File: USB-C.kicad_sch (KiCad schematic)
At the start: 38 parts, among them IC2 TPS2557QDRBTQ1, IC5 TPS2557QDRBTQ1, IC7 TPS2557QDRBTQ1, J10 USB_C_Receptacle, J5 USB_C_Receptacle_USB2.0_16P, J7 USB_C_Receptacle_USB2.0_16P, U2 TPD1E05U06DYA, U3 TPD1E05U06DYA, U4 TPD1E05U06DYA

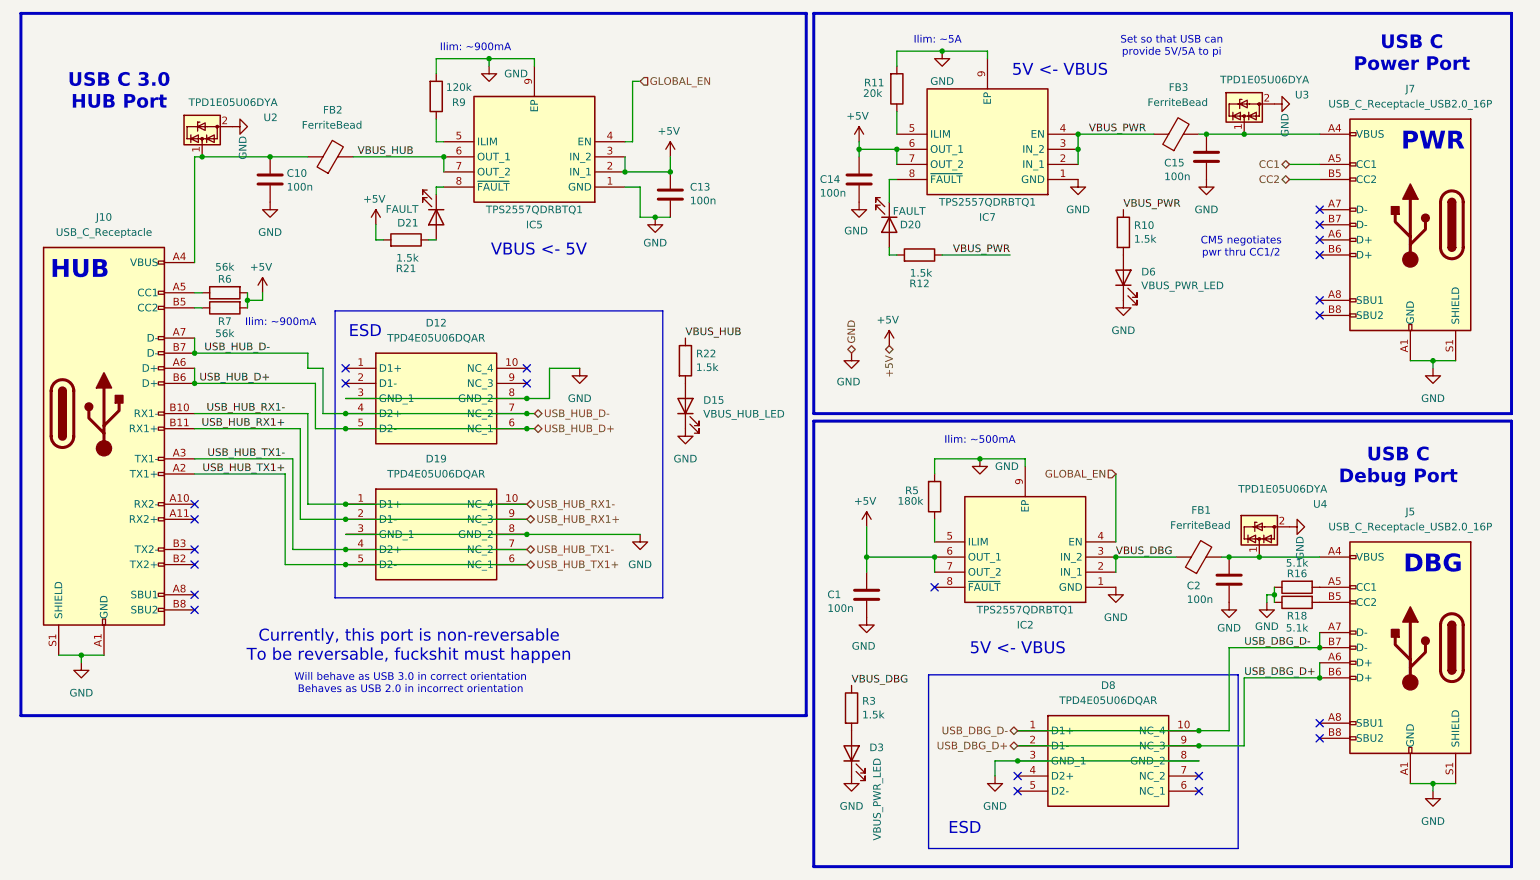
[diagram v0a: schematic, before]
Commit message: my life could not be worse right now
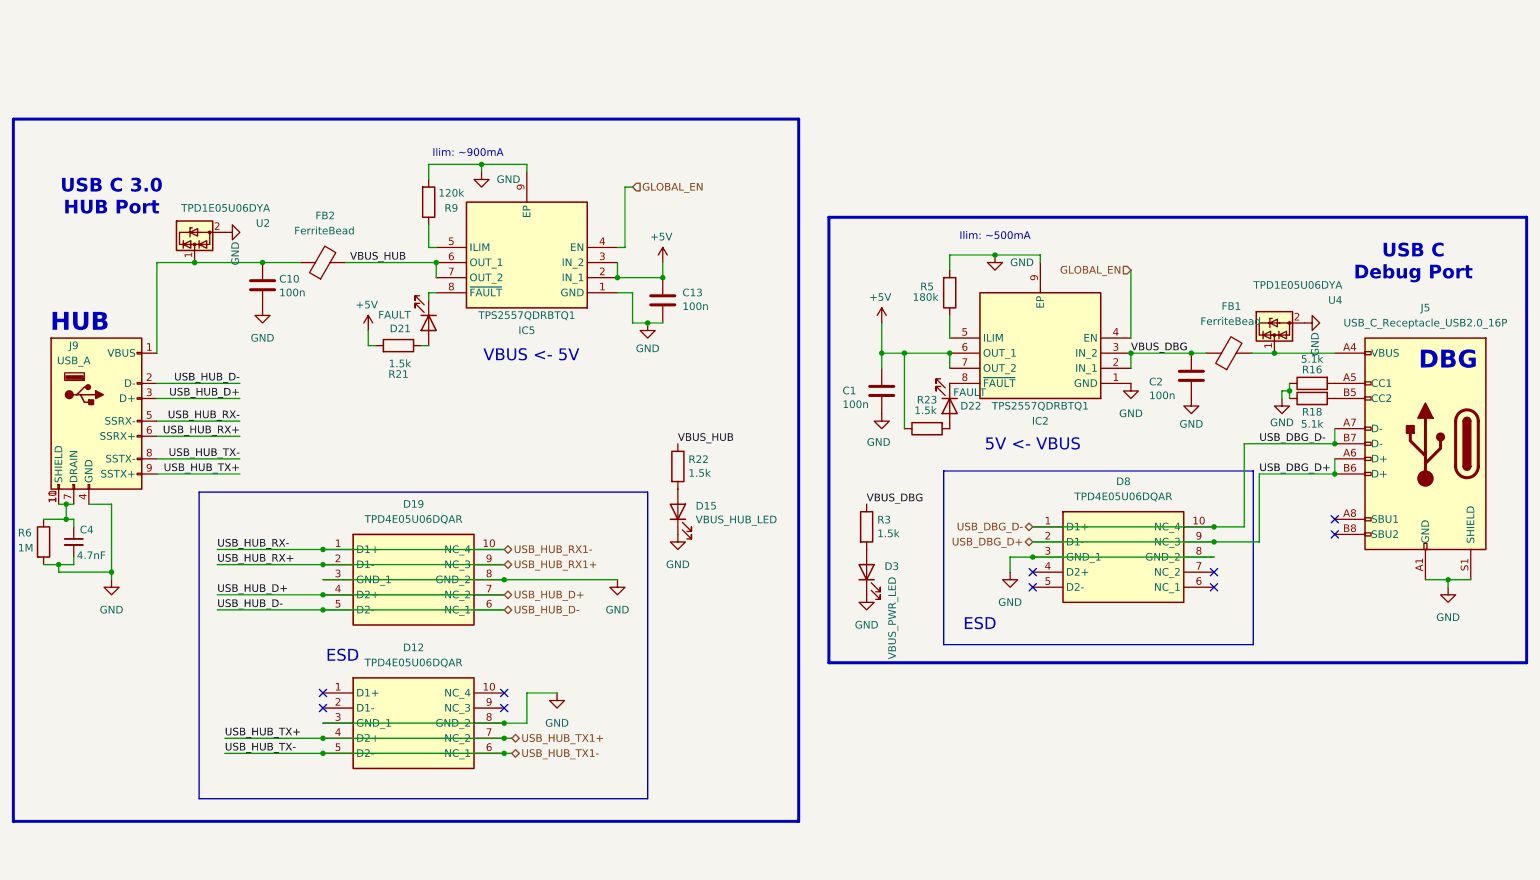
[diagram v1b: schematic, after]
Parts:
- removed C14, C15: 100n, Capacitor_SMD:C_0603_1608Metric_Pad1.08x0.95mm_HandSolder, symbol Device:C
- removed D20: FAULT, LED_SMD:LED_0603_1608Metric_Pad1.05x0.95mm_HandSolder, symbol Device:LED
- removed D6: VBUS_PWR_LED, LED_SMD:LED_0603_1608Metric_Pad1.05x0.95mm_HandSolder, symbol Device:LED
- removed FB3: FerriteBead, Inductor_SMD:L_1206_3216Metric, symbol Device:FerriteBead
- removed IC7: TPS2557QDRBTQ1, Controls_Pi:SON65P300X300X100-9N-D, symbol TPS2557QDRBTQ1:TPS2557QDRBTQ1
- removed J10: USB_C_Receptacle, Controls_Pi:CONN_221608-0001_MOL, symbol Connector:USB_C_Receptacle
- removed J7: USB_C_Receptacle_USB2.0_16P, Controls_Pi:2193200001, symbol Connector:USB_C_Receptacle_USB2.0_16P
- removed R10, R12: 1.5k, Resistor_SMD:R_0603_1608Metric_Pad0.98x0.95mm_HandSolder, symbol Device:R
- removed R11: 20k, Resistor_SMD:R_0603_1608Metric_Pad0.98x0.95mm_HandSolder, symbol Device:R
- removed R7: 56k, Resistor_SMD:R_0603_1608Metric_Pad0.98x0.95mm_HandSolder, symbol Device:R
- removed U3: TPD1E05U06DYA, Diode_SMD:D_SOD-523, symbol Power_Protection:TPD1E05U06DYA
- added C4: 4.7nF, Capacitor_SMD:C_0603_1608Metric_Pad1.08x0.95mm_HandSolder, symbol Device:C_Small
- added D22: FAULT, LED_SMD:LED_0603_1608Metric_Pad1.05x0.95mm_HandSolder, symbol Device:LED
- added J9: USB_A, Controls_Pi:CONN_484050003_MOL, symbol Connector:USB_A
- added R23: 1.5k, Resistor_SMD:R_0603_1608Metric_Pad0.98x0.95mm_HandSolder, symbol Device:R
- R6: value 56k -> 1M
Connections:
- net +5V: now also R23.1; no longer R6.2
- net GND: now also R6.2, C4.2, J9.4 (GND)
- net USB_HUB_D+: now also D19.4 (D2+), D19.7 (NC_2), J9.3 (D+); no longer D12.5 (D2-), D12.6 (NC_1)
- net USB_HUB_D-: now also D19.5 (D2-), D19.6 (NC_1), J9.2 (D-); no longer D12.4 (D2+), D12.7 (NC_2)
- net USB_HUB_RX1+: now also J9.6 (SSRX+)
- net USB_HUB_RX1-: now also J9.5 (SSRX-)
- net USB_HUB_TX1+: now also D12.4 (D2+), D12.7 (NC_2), J9.9 (SSTX+); no longer D19.5 (D2-), D19.6 (NC_1)
- net USB_HUB_TX1-: now also D12.5 (D2-), D12.6 (NC_1), J9.8 (SSTX-); no longer D19.4 (D2+), D19.7 (NC_2)
- net VBUS_DBG: now also C2.1
- net at C10.1, FB2.1, U2.1 (I/O): now also J9.1 (VBUS)
- net at FB1.2, J5.A4 (VBUS), J5.A9 (VBUS)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: no longer C2.1
- net at R6.1: now also C4.1, J9.10 (SHIELD), J9.11 (SHIELD), J9.7 (DRAIN)
- net at IC2.8 (~{FAULT}): now also D22.1 (K)
- new net: D22.2 (A), R23.2
- no-connect marks 23 -> 10
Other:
- note removed: "CM5 negotiates pwr thru CC1/2"
- note removed: "Currently, this port is non-reversable To be reversable, fuckshit must happen"
- note removed: "Ilim: ~5A"
- note removed: "PWR"
- note removed: "Set so that USB can provide 5V/5A to pi"
- note removed: "USB C Power Port"
- note removed: "Will behave as USB 3.0 in correct orientation Behaves as USB 2.0 in incorrect orientation"
- moved on the sheet: C1, C10, C13, C2, D12, D15, D19, D21, D3, D8, FB1, FB2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

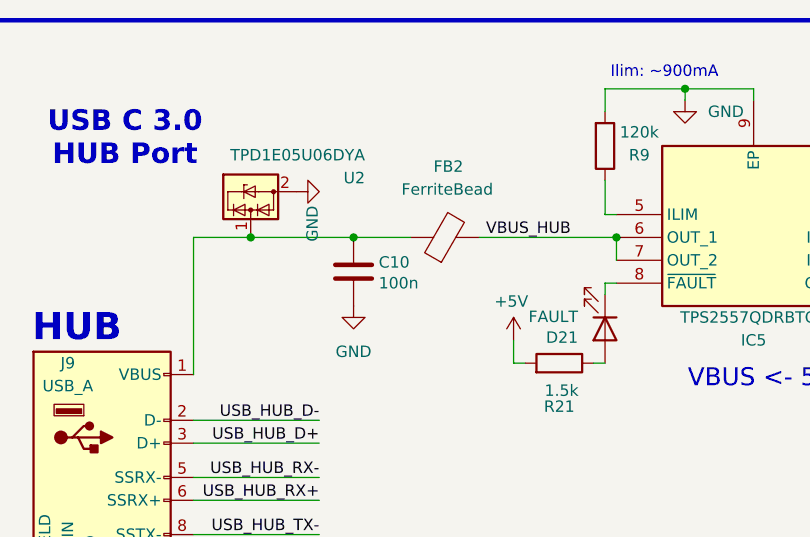
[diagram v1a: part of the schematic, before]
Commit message: frink2
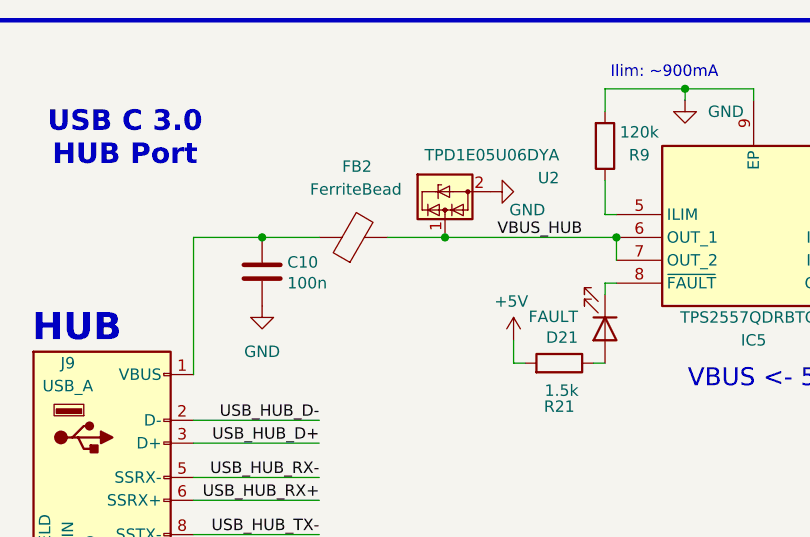
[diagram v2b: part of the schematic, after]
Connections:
- net VBUS_HUB: now also U2.1 (I/O)
- net at C10.1, FB2.1, J9.1 (VBUS): no longer U2.1 (I/O)
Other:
- moved on the sheet: C10, FB2, U2
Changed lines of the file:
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@@
 	)
 	(junction
+		(at 73.66 57.15)
+		(diameter 0)
+		(color 0 0 0 0)
+	)
+	(junction
 		(at 233.68 72.39)
 		(diameter 0)
@@
 	)
 	(junction
-		(at 52.07 57.15)
-		(diameter 0)
-		(color 0 0 0 0)
-	)
-	(junction
 		(at 73.66 107.95)
 		(diameter 0)
@@
 	)
 	(junction
-		(at 63.5 57.15)
+		(at 53.34 57.15)
 		(diameter 0)
 		(color 0 0 0 0)
@@
 	(wire
 		(pts
-			(xy 52.07 57.15) (xy 63.5 57.15)
+			(xy 45.72 57.15) (xy 53.34 57.15)
 		)
 		(stroke
@@
 	(wire
 		(pts
-			(xy 63.5 57.15) (xy 69.85 57.15)
+			(xy 53.34 57.15) (xy 59.69 57.15)
 		)
 		(stroke
@@
 	(wire
 		(pts
+			(xy 73.66 57.15) (xy 92.71 57.15)
+		)
+		(stroke
+			(width 0)
+			(type default)
+		)
+	)
+	(wire
+		(pts
 			(xy 231.14 92.71) (xy 231.14 104.14)
 		)
@@
 	(wire
 		(pts
-			(xy 77.47 57.15) (xy 92.71 57.15)
+			(xy 67.31 57.15) (xy 73.66 57.15)
 		)
 		(stroke
@@
 	(wire
 		(pts
-			(xy 45.72 57.15) (xy 52.07 57.15)
-		)
-		(stroke
-			(width 0)
-			(type default)
-		)
-	)
-	(wire
-		(pts
 			(xy 100.33 41.91) (xy 100.33 40.64)
 		)
@@
 	)
 	(label "VBUS_HUB"
-		(at 87.63 57.15 180)
+		(at 88.9 57.15 180)
 		(effects
 			(font
@@
 	(symbol
 		(lib_id "power:GND")
-		(at 63.5 64.77 0)
+		(at 53.34 64.77 0)
 		(unit 1)
 		(exclude_from_sim no)
@@
 		(fields_autoplaced yes)
 		(property "Reference" "#PWR024"
-			(at 63.5 71.12 0)
+			(at 53.34 71.12 0)
 			(effects
 				(font
@@
 		)
 		(property "Value" "GND"
-			(at 63.5 69.85 0)
+			(at 53.34 69.85 0)
 			(effects
 				(font
@@
 		)
 		(property "Footprint" ""
-			(at 63.5 64.77 0)
+			(at 53.34 64.77 0)
 			(effects
 				(font
@@
 		)
 		(property "Datasheet" ""
-			(at 63.5 64.77 0)
+			(at 53.34 64.77 0)
 			(effects
 				(font
@@
 		)
 		(property "Description" "Power symbol creates a global label with name \"GND\" , ground"
-			(at 63.5 64.77 0)
+			(at 53.34 64.77 0)
 			(effects
 				(font
@@
 	(symbol
 		(lib_id "Device:FerriteBead")
-		(at 73.66 57.15 90)
+		(at 63.5 57.15 90)
 		(unit 1)
 		(exclude_from_sim no)
@@
 		(dnp no)
 		(property "Reference" "FB2"
-			(at 75.692 49.276 90)
+			(at 65.532 49.276 90)
 			(effects
 				(font
@@
 		)
 		(property "Value" "FerriteBead"
-			(at 73.914 51.816 90)
+			(at 63.754 51.816 90)
 			(effects
 				(font
@@
 		)
 		(property "Footprint" "Inductor_SMD:L_1206_3216Metric"
-			(at 73.66 58.928 90)
+			(at 63.5 58.928 90)
 			(effects
 				(font
@@
 		)
 		(property "Datasheet" "https://www.te.com/commerce/DocumentDelivery/DDEController?Action=srchrtrv&DocNm=1773178-3&DocType=Data%20Sheet&DocLang=English&DocFormat=pdf&PartCntxt=2-2176745-0"
-			(at 73.66 57.15 0)
+			(at 63.5 57.15 0)
 			(effects
 				(font
@@
 		)
 		(property "Description" "Ferrite bead"
-			(at 73.66 57.15 0)
+			(at 63.5 57.15 0)
 			(effects
 				(font
@@
 		)
 		(property "P/N" "BMC-Q2CY0220H "
-			(at 73.66 57.15 0)
+			(at 63.5 57.15 0)
 			(effects
 				(font
@@
 	(symbol
 		(lib_id "power:GND")
-		(at 57.15 52.07 90)
+		(at 78.74 52.07 90)
 		(unit 1)
 		(exclude_from_sim no)
@@
 		(dnp no)
 		(property "Reference" "#PWR0120"
-			(at 63.5 52.07 0)
+			(at 85.09 52.07 0)
 			(effects
 				(font
@@
 		)
 		(property "Value" "GND"
-			(at 58.928 55.626 0)
+			(at 82.804 54.102 90)
 			(effects
 				(font
@@
 		)
 		(property "Footprint" ""
-			(at 57.15 52.07 0)
+			(at 78.74 52.07 0)
 			(effects
 				(font
@@
 		)
 		(property "Datasheet" ""
-			(at 57.15 52.07 0)
+			(at 78.74 52.07 0)
 			(effects
 				(font
@@
 		)
 		(property "Description" "Power symbol creates a global label with name \"GND\" , ground"
-			(at 57.15 52.07 0)
+			(at 78.74 52.07 0)
 			(effects
 				(font
@@
 	(symbol
 		(lib_id "Power_Protection:TPD1E05U06DYA")
-		(at 52.07 52.07 0)
+		(at 73.66 52.07 0)
 		(unit 1)
 		(exclude_from_sim no)
@@
 		(dnp no)
 		(property "Reference" "U2"
-			(at 64.77 50.546 0)
+			(at 86.36 50.546 0)
 			(effects
 				(font
@@
 		)
 		(property "Value" "TPD1E05U06DYA"
-			(at 64.77 48.006 0)
+			(at 86.36 48.006 0)
 			(effects
 				(font
@@
 		)
 		(property "Footprint" "Diode_SMD:D_SOD-523"
-			(at 54.61 56.515 0)
+			(at 76.2 56.515 0)
 			(effects
 				(font
@@
 		)
 		(property "Datasheet" "https://www.ti.com/lit/ds/symlink/tpd1e05u06.pdf"
-			(at 54.61 58.42 0)
+			(at 76.2 58.42 0)
 			(effects
 				(font
@@
 		)
 		(property "Description" "1-Channel ESD Protection for Super-Speed USB 3.0 Interface, SOD-523"
-			(at 52.07 52.07 0)
+			(at 73.66 52.07 0)
 			(effects
 				(font
@@
 	(symbol
 		(lib_id "Device:C")
-		(at 63.5 60.96 0)
+		(at 53.34 60.96 0)
 		(unit 1)
 		(exclude_from_sim no)
@@
 		(dnp no)
 		(property "Reference" "C10"
-			(at 66.294 59.9186 0)
+			(at 56.134 59.9186 0)
 			(effects
 				(font
@@
 		)
 		(property "Value" "100n"
-			(at 66.294 62.23 0)
+			(at 56.134 62.23 0)
 			(effects
 				(font
@@
 		)
 		(property "Footprint" "Capacitor_SMD:C_0603_1608Metric_Pad1.08x0.95mm_HandSolder"
-			(at 64.4652 64.77 0)
+			(at 54.3052 64.77 0)
 			(effects
 				(font
@@
 		)
 		(property "Datasheet" "https://content.kemet.com/datasheets/KEM_C1002_X7R_SMD.pdf"
-			(at 63.5 60.96 0)
+			(at 53.34 60.96 0)
 			(effects
 				(font
@@
 		)
 		(property "Description" "Unpolarized capacitor"
-			(at 63.5 60.96 0)
+			(at 53.34 60.96 0)
 			(effects
 				(font
@@
 		)
 		(property "P/N" "C0805C104M5RACTU"
-			(at 63.5 60.96 0)
+			(at 53.34 60.96 0)
 			(effects
 				(font

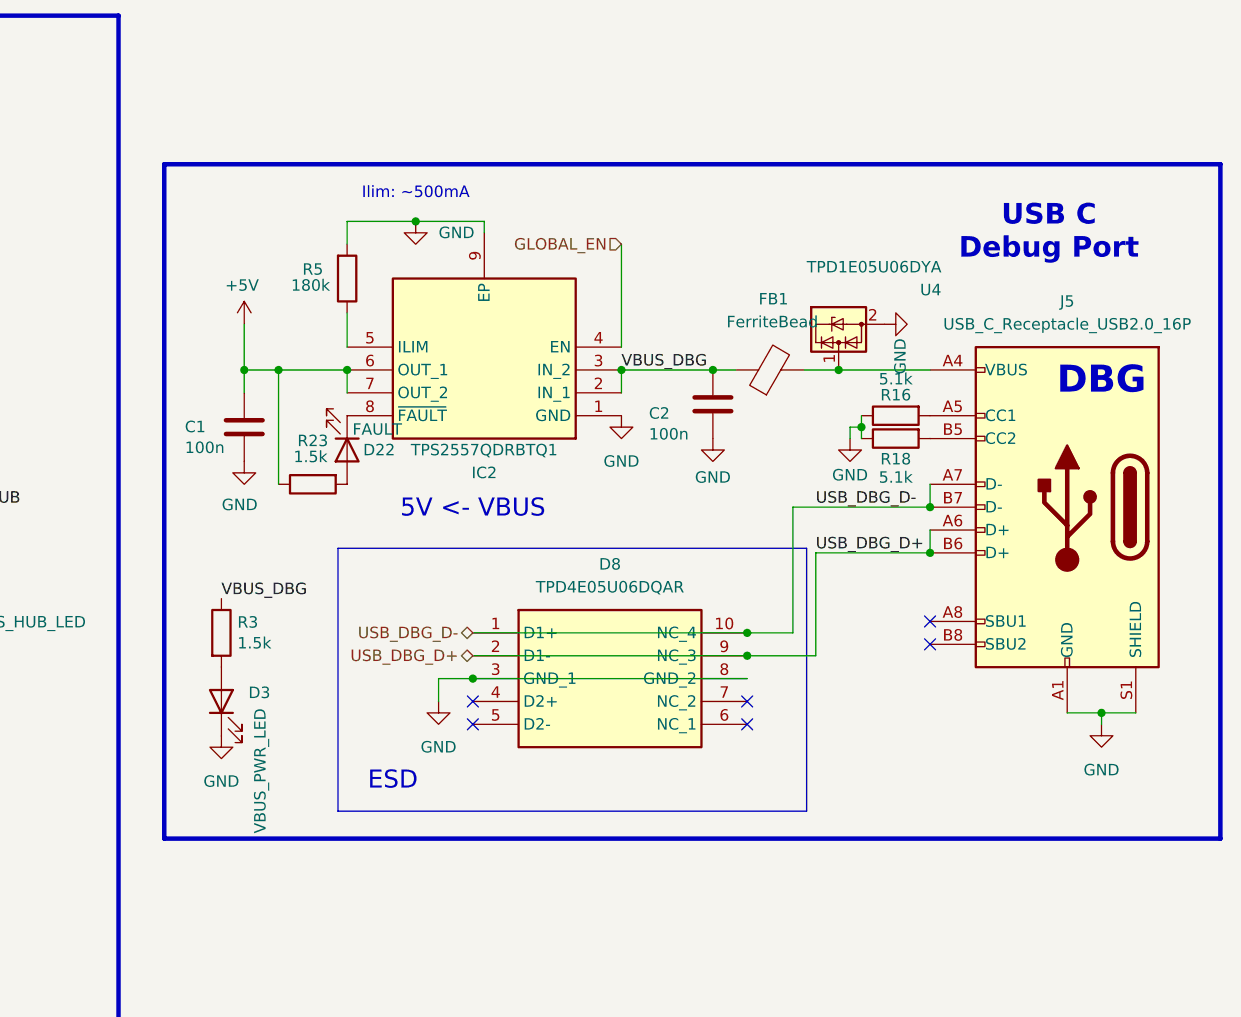
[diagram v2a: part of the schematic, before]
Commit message: lak
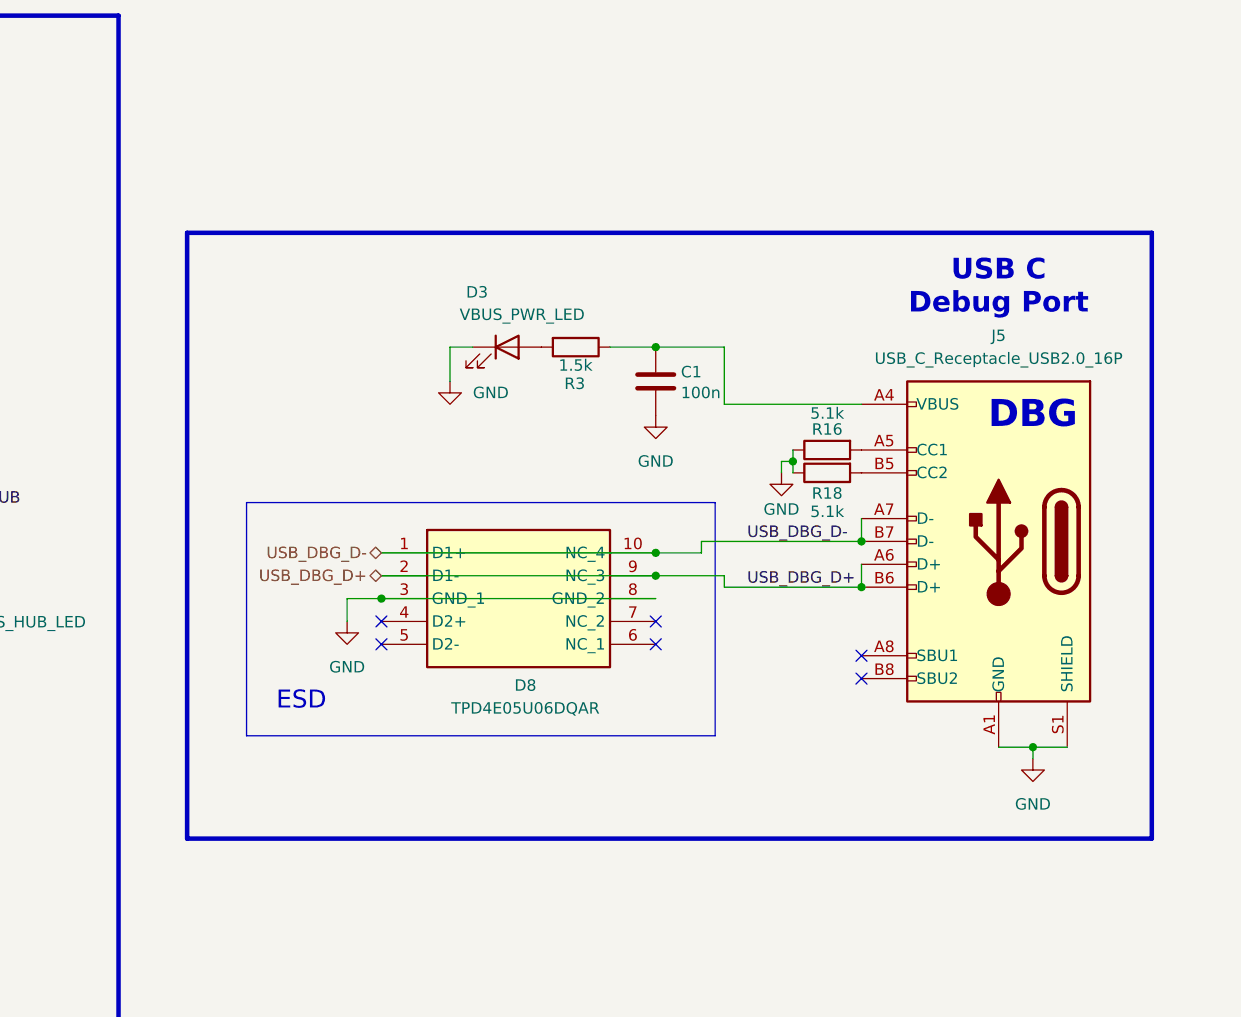
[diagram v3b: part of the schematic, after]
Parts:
- removed C2: 100n, Capacitor_SMD:C_0603_1608Metric_Pad1.08x0.95mm_HandSolder, symbol Device:C
- removed D22: FAULT, LED_SMD:LED_0603_1608Metric_Pad1.05x0.95mm_HandSolder, symbol Device:LED
- removed FB1: FerriteBead, Inductor_SMD:L_1206_3216Metric, symbol Device:FerriteBead
- removed IC2: TPS2557QDRBTQ1, Controls_Pi:SON65P300X300X100-9N-D, symbol TPS2557QDRBTQ1:TPS2557QDRBTQ1
- removed R23: 1.5k, Resistor_SMD:R_0603_1608Metric_Pad0.98x0.95mm_HandSolder, symbol Device:R
- removed R5: 180k, Resistor_SMD:R_0603_1608Metric_Pad0.98x0.95mm_HandSolder, symbol Device:R
- removed U4: TPD1E05U06DYA, Diode_SMD:D_SOD-523, symbol Power_Protection:TPD1E05U06DYA
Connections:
- net VBUS_DBG is gone; now on an unnamed net: R3.1
- net +5V: no longer C1.1
- net at J5.A4 (VBUS), J5.A9 (VBUS), J5.B4 (VBUS)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: now also C1.1
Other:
- note removed: "5V <- VBUS"
- note removed: "Ilim: ~500mA"
- moved on the sheet: D3, D8, J5, R16, R18, R3
